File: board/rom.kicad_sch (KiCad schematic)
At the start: 4 parts, among them U2 ROM LO, U3 ROM HI

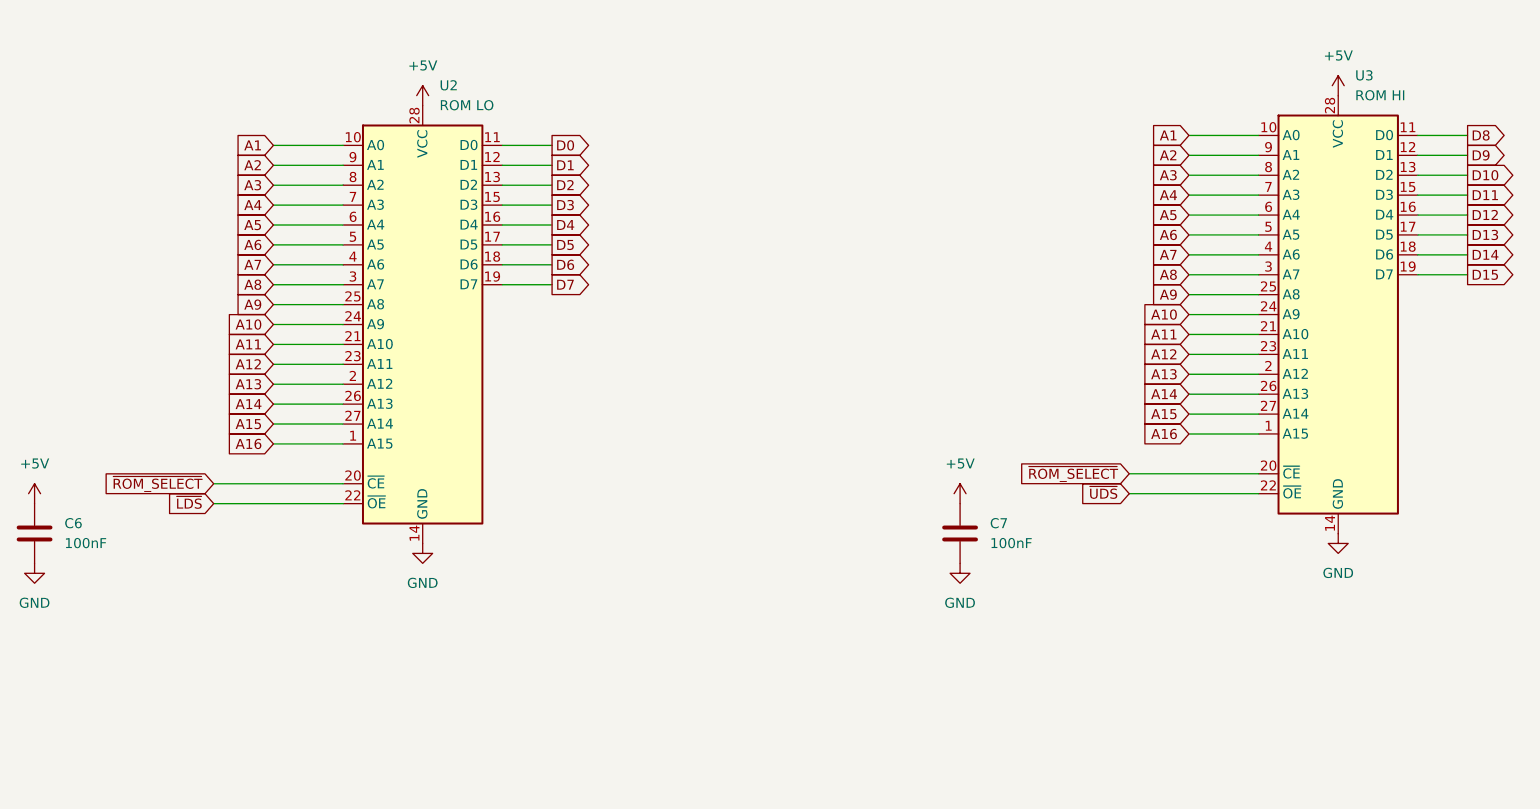
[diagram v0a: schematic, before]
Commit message: checkpoint
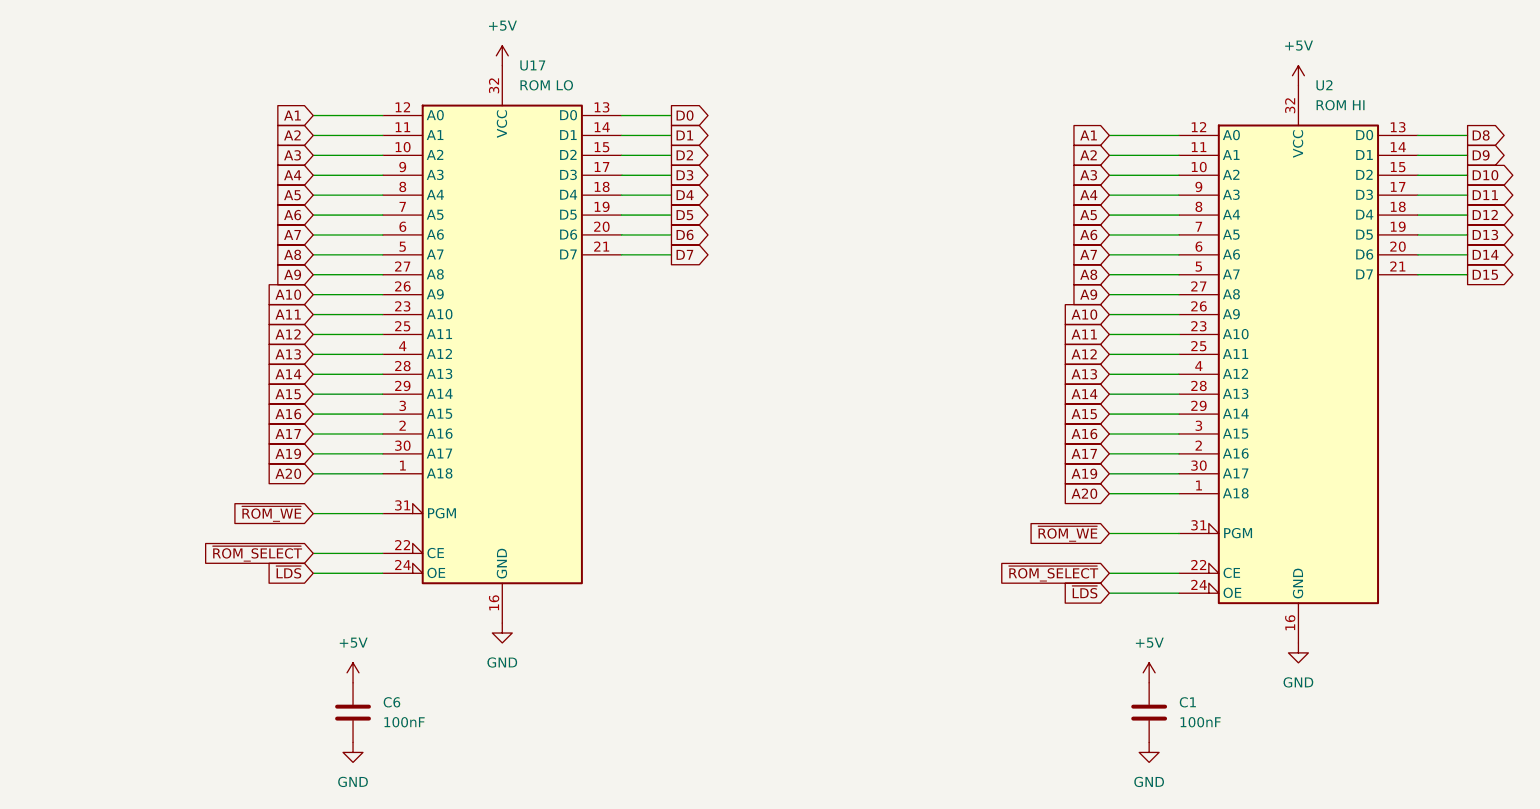
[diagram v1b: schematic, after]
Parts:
- removed C7: 100nF, Capacitor_THT:C_Disc_D5.0mm_W2.5mm_P5.00mm, symbol Device:C
- removed U2: ROM LO, Package_DIP:DIP-28_W15.24mm, symbol Memory_EPROM:27C512
- removed U3: ROM HI, Package_DIP:DIP-28_W15.24mm, symbol Memory_EPROM:27C512
- added C1: 100nF, Capacitor_THT:C_Disc_D5.0mm_W2.5mm_P5.00mm, symbol Device:C
- added U17: ROM LO, symbol Memory_Flash:SST39SF040
- added U2: ROM HI, symbol Memory_Flash:SST39SF040
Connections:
- net +5V: now also C1.1, U17.32 (VCC), U2.32 (VCC)
- net A1: now also U17.12 (A0), U2.12 (A0)
- net A10: now also U17.26 (A9), U2.26 (A9)
- net A11: now also U17.23 (A10), U2.23 (A10)
- net A12: now also U17.25 (A11), U2.25 (A11)
- net A13: now also U17.4 (A12), U2.4 (A12)
- net A14: now also U17.28 (A13), U2.28 (A13)
- net A15: now also U17.29 (A14), U2.29 (A14)
- net A16: now also U17.3 (A15), U2.3 (A15)
- net A2: now also U17.11 (A1), U2.11 (A1)
- net A3: now also U17.10 (A2), U2.10 (A2)
- net A4: now also U17.9 (A3), U2.9 (A3)
- net A5: now also U17.8 (A4), U2.8 (A4)
- net A6: now also U17.7 (A5), U2.7 (A5)
- net A7: now also U17.6 (A6), U2.6 (A6)
- net A8: now also U17.5 (A7), U2.5 (A7)
- net A9: now also U17.27 (A8), U2.27 (A8)
- net D0: now also U17.13 (D0)
- net D1: now also U17.14 (D1)
- net D10: now also U2.15 (D2)
- net D11: now also U2.17 (D3)
- net D12: now also U2.18 (D4)
- net D13: now also U2.19 (D5)
- net D14: now also U2.20 (D6)
- net D15: now also U2.21 (D7)
- net D2: now also U17.15 (D2)
- net D3: now also U17.17 (D3)
- net D4: now also U17.18 (D4)
- net D5: now also U17.19 (D5)
- net D6: now also U17.20 (D6)
- net D7: now also U17.21 (D7)
- net D8: now also U2.13 (D0)
- net D9: now also U2.14 (D1)
- net GND: now also C1.2, U17.16 (GND), U2.16 (GND)
- net ~{LDS}: now also U17.24 (OE), U2.24 (OE)
- net ~{ROM_SELECT}: now also U17.22 (CE), U2.22 (CE)
- new net A17: U17.2 (A16), U2.2 (A16)
- new net A19: U17.30 (A17), U2.30 (A17)
- new net A20: U17.1 (A18), U2.1 (A18)
- new net ~{ROM_WE}: U17.31 (PGM), U2.31 (PGM)
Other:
- moved on the sheet: C6
